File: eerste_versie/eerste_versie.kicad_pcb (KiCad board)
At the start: 2 copper layers, 12 parts, among them U1 ESP32-WROOM-32U, U2 AMS1117-3.3, X1 DG3XX-02-5.0

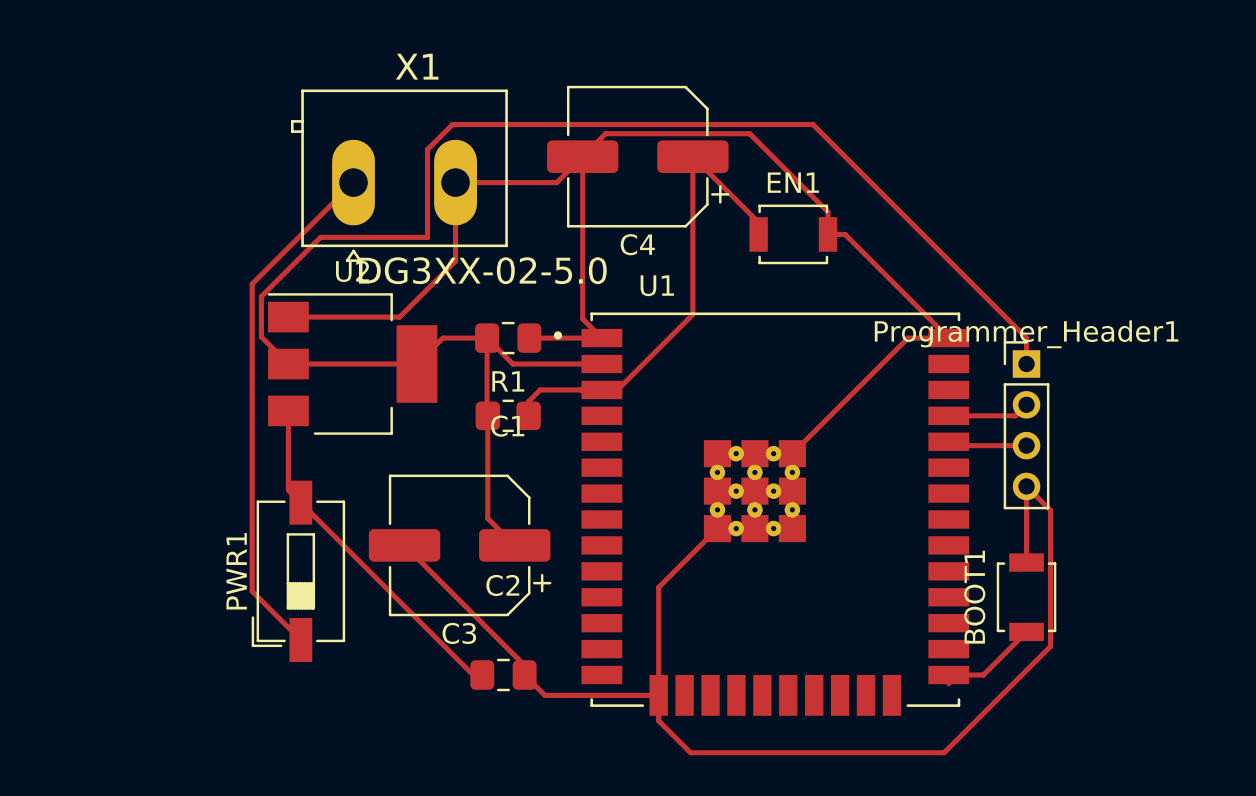
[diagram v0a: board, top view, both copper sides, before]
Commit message: tweede versie
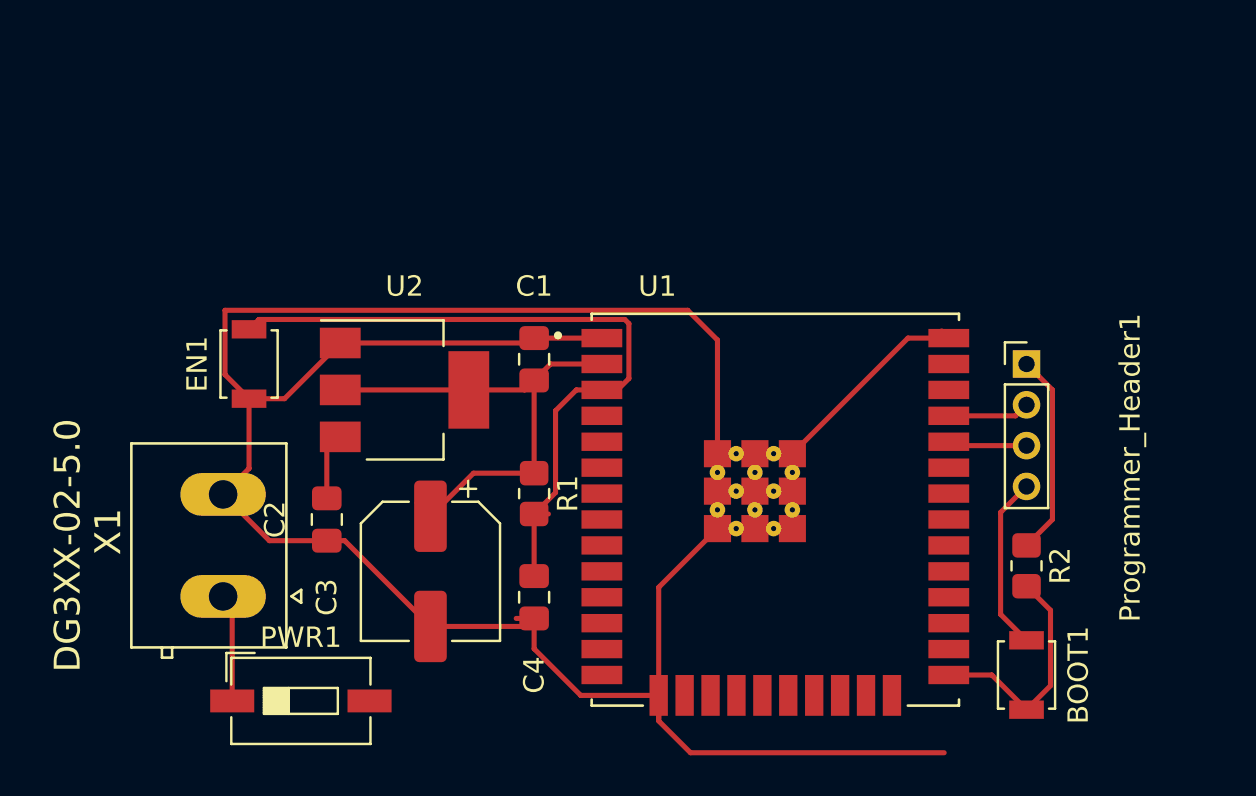
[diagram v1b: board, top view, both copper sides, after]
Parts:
- added R2: 10k, Resistor_SMD:R_0805_2012Metric_Pad1.20x1.40mm_HandSolder, F.Cu at (152.4, 117.8)
- C4: value 47u -> 1u; footprint Capacitor_SMD:CP_Elec_6.3x3 -> Capacitor_SMD:C_0805_2012Metric_Pad1.18x1.45mm_HandSolder
- moved EN1 27.4 mm to (114.3, 108.0), turned to 270 degrees
- moved C4 22.2 mm to (128.3, 119.4), turned to 270 degrees
- moved X1 19.9 mm to (113.0, 116.8), turned to 90 degrees
- moved C2 11.5 mm to (118.1, 115.6), turned to 270 degrees
- moved PWR1 6.35 mm to (116.8, 124.5), turned to 0 degrees
- moved R1 4.02 mm to (128.3, 114.3), turned to 270 degrees
- moved BOOT1 3.81 mm to (152.4, 123.2)
- moved U2 2.84 mm to (121.9, 109.2)
- moved C3 1.91 mm to (123.2, 118.1), turned to 270 degrees
- moved C1 1.64 mm to (128.3, 107.7), turned to 270 degrees
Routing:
- net VDD33: track 80.1 -> 35.1 mm
- net Net-(PWR1-Pad1): track 25.5 -> 5.30 mm
- net Net-(C2-Pad1): track 17.1 -> 3.89 mm
- net Net-(C4-Pad1): track 24.4 -> 35.1 mm
- net Net-(BOOT1-Pad1): track 6.64 -> 12.3 mm
- net GND: track 150.9 -> 154.2 mm
